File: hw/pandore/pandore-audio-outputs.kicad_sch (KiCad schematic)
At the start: 2 parts, among them J12 TRS, J7 TRS

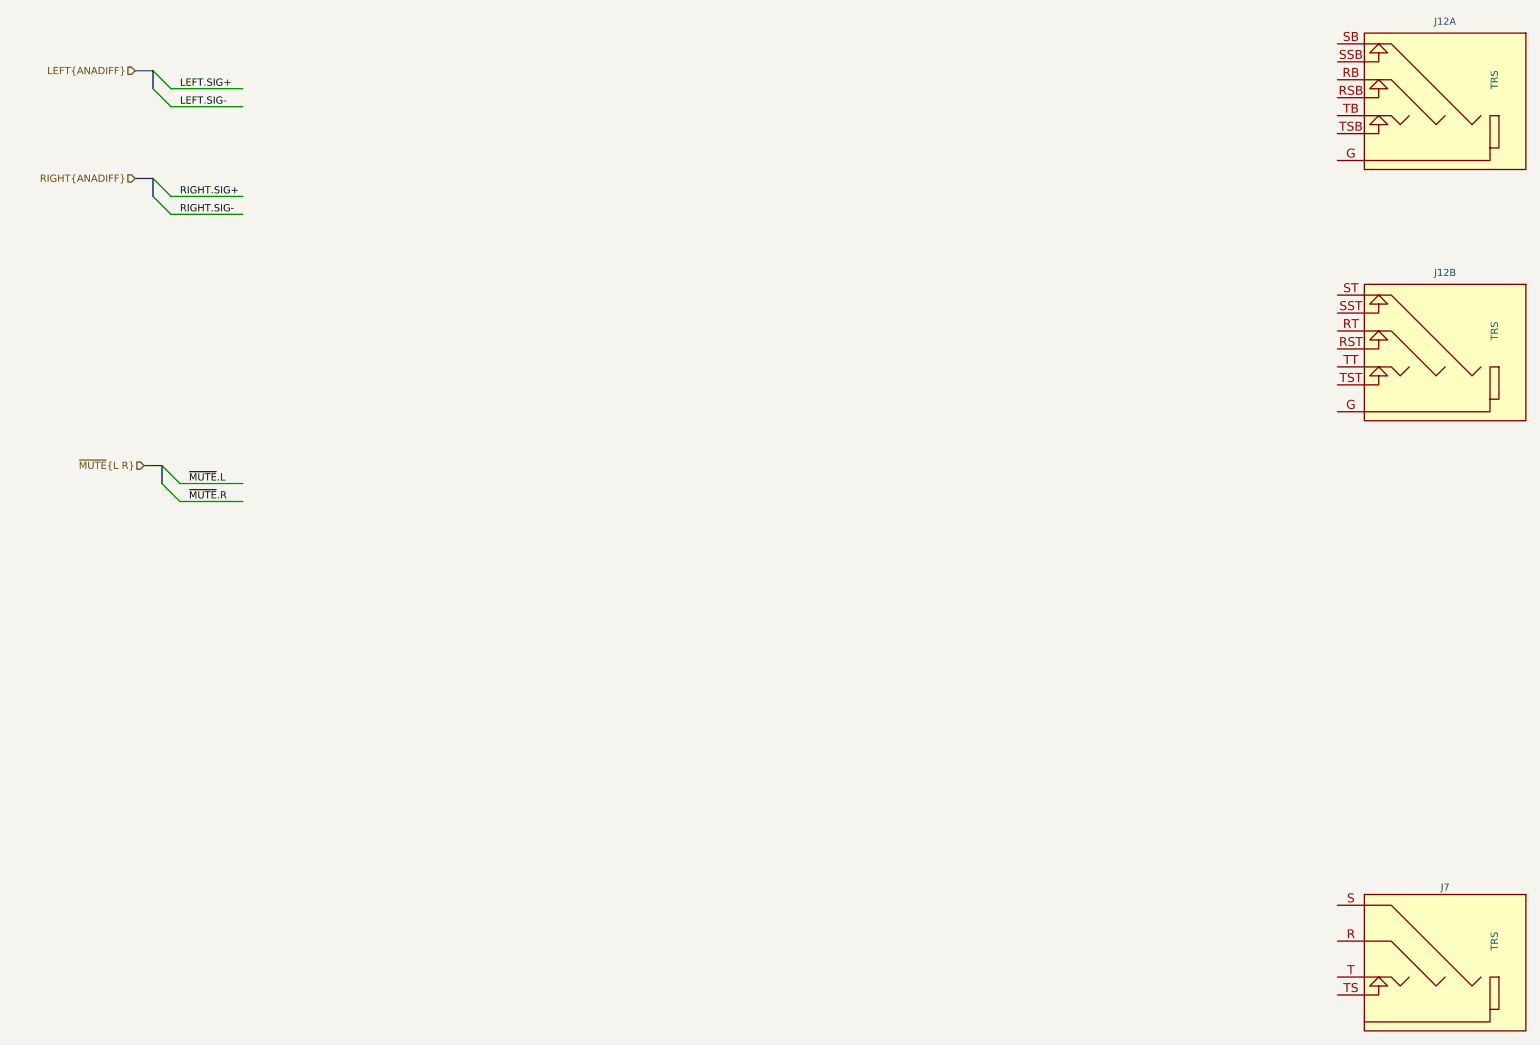
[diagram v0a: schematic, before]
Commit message: lots of work done all around
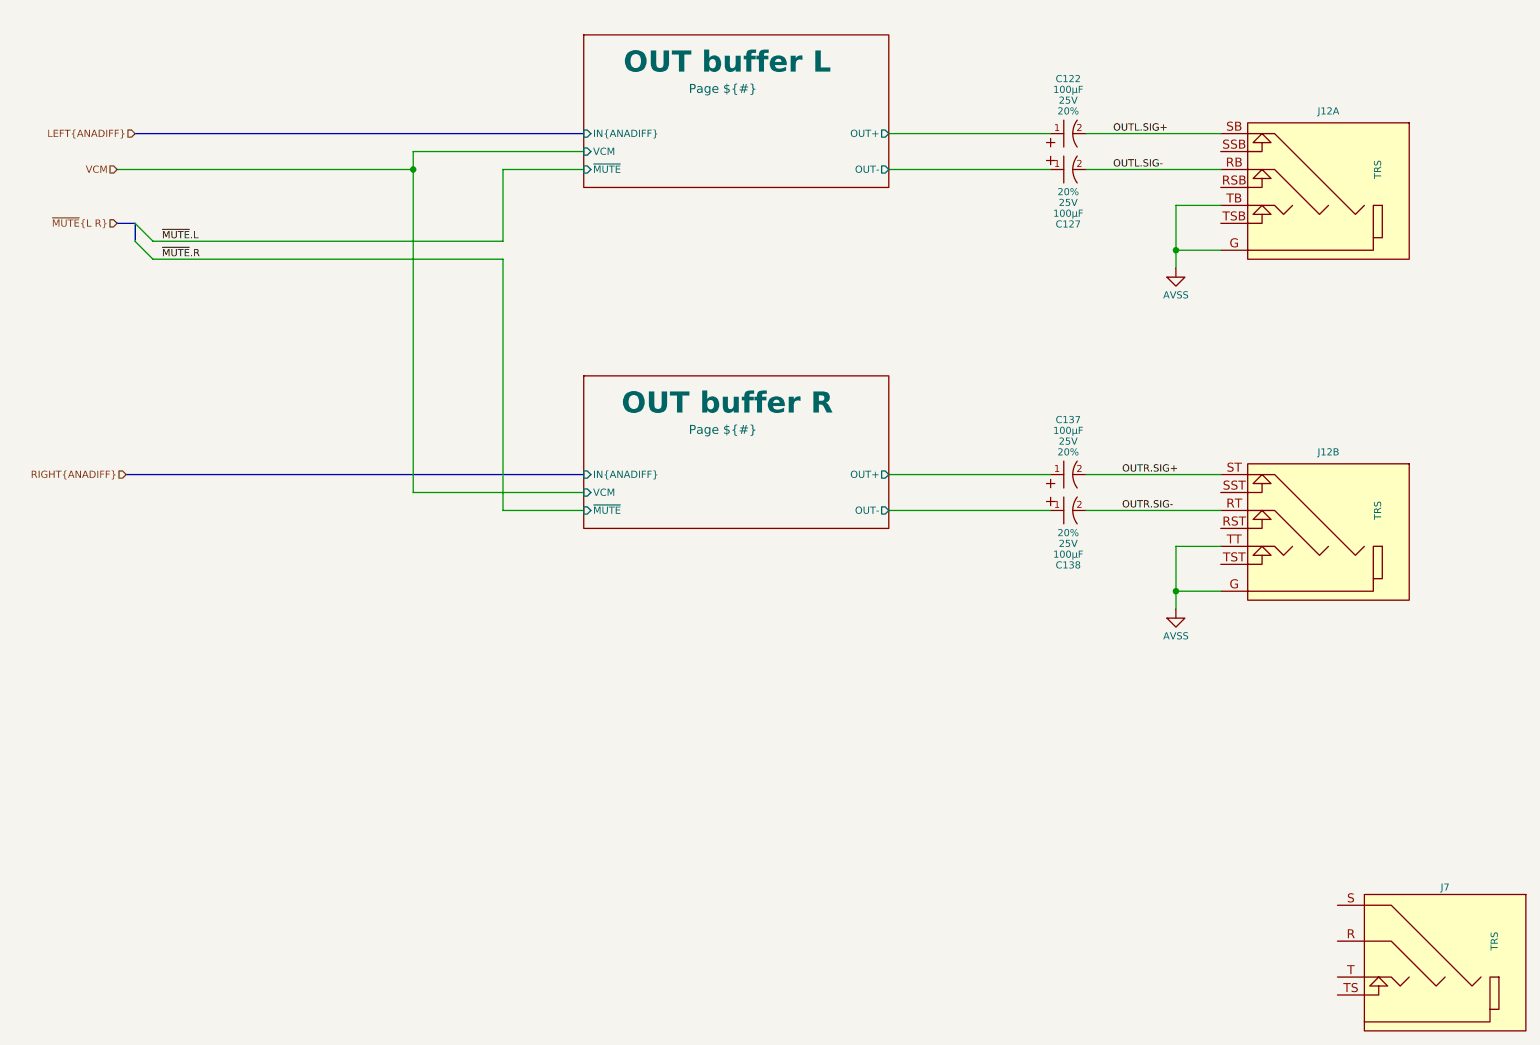
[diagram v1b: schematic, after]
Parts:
- added C122, C127, C137, C138: ${Capacitance}, ${Voltage}, ${Tolerance}, reekilib_cap:CAPAE630Xxxx, symbol reekilib_cap:cap_pol
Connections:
- net AVSS: now reaches J12.G
- net AVSS: now also J12.G, J12.TB, J12.TT
- net OUTR.SIG-: now reaches J12.RT
- net OUTR.SIG-: now also C138.2 (-)
- net OUTR.SIG+: now reaches J12.ST
- net OUTR.SIG+: now also C137.2 (-)
- net OUTL.SIG-: now reaches J12.RB
- net OUTL.SIG-: now also C127.2 (-)
- net OUTL.SIG+: now reaches J12.SB
- net OUTL.SIG+: now also C122.2 (-)
- new net OUT buffer L/OUT+: C122.1 (+)
- new net OUT buffer L/OUT-: C127.1 (+)
- new net OUT buffer R/OUT+: C137.1 (+)
- new net OUT buffer R/OUT-: C138.1 (+)
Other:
- added sheet OUT buffer L (pandore-audio-outbuf.kicad_sch)
- added sheet OUT buffer R (pandore-audio-outbuf.kicad_sch)
- moved on the sheet: J12A, J12B
